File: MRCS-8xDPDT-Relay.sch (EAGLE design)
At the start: 19 parts, among them CON1 CONNECTOR-M10LOCK, K1 RELAY-G2R2, K2 RELAY-G2R2, K3 RELAY-G2R2, K4 RELAY-G2R2, K5 RELAY-G2R2, K6 RELAY-G2R2, K7 RELAY-G2R2, K8 RELAY-G2R2

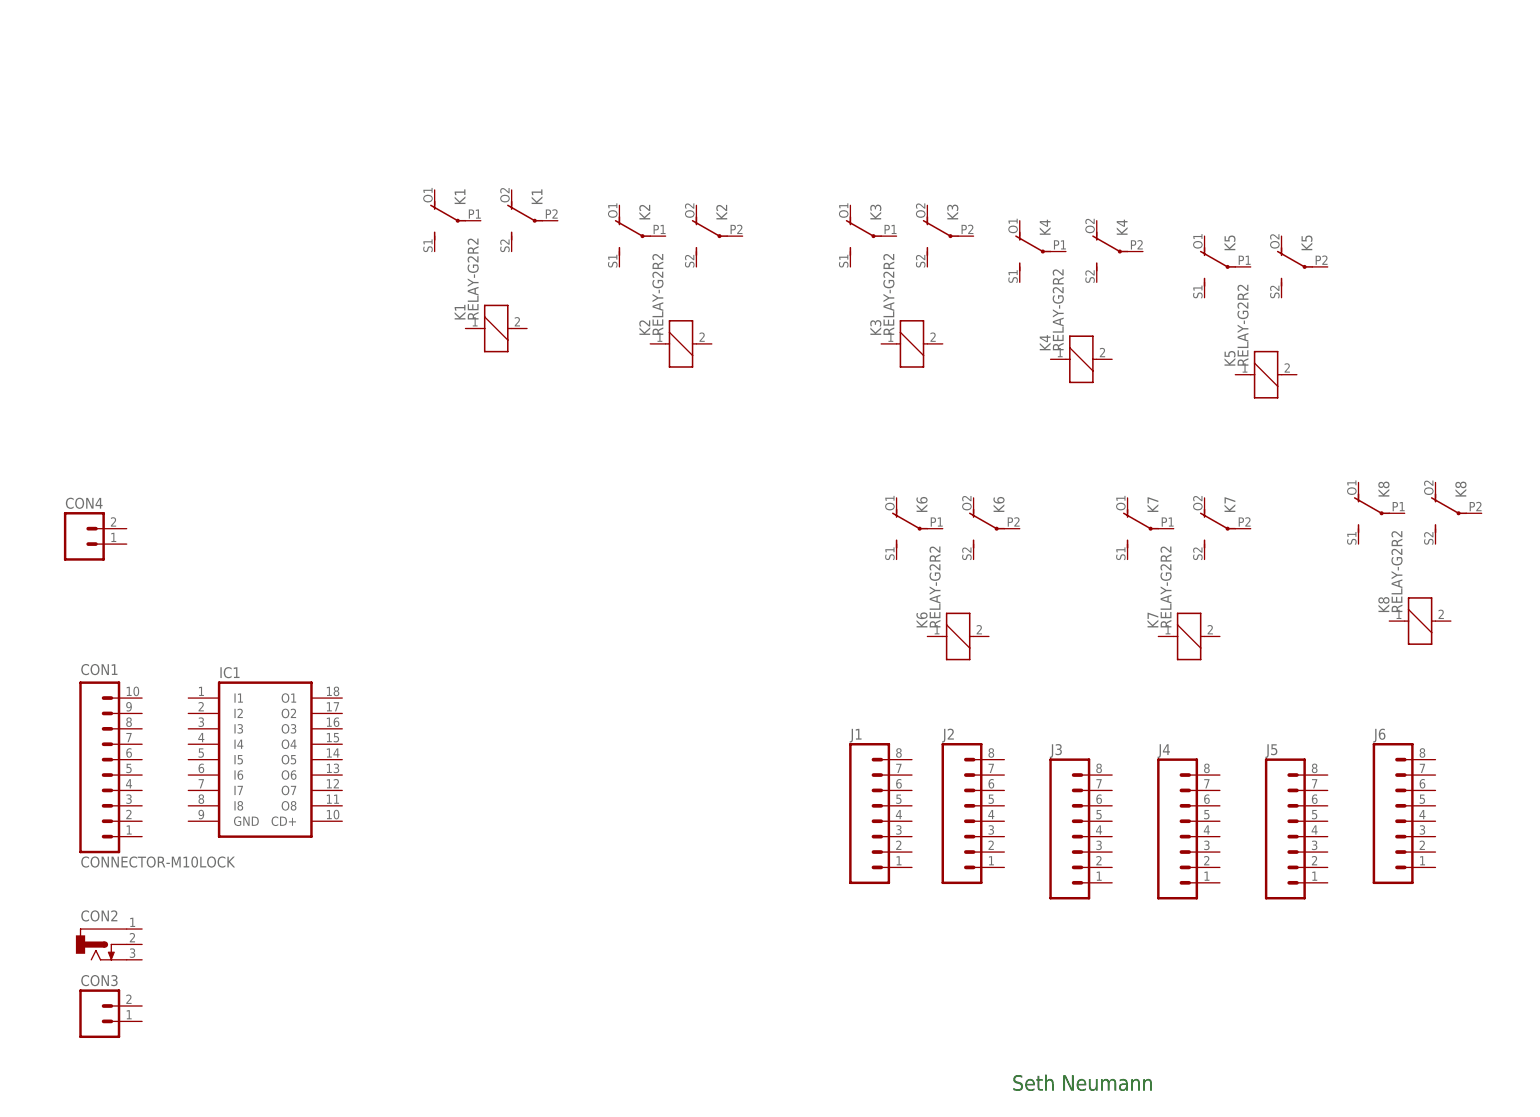
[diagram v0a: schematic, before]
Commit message: early doodling
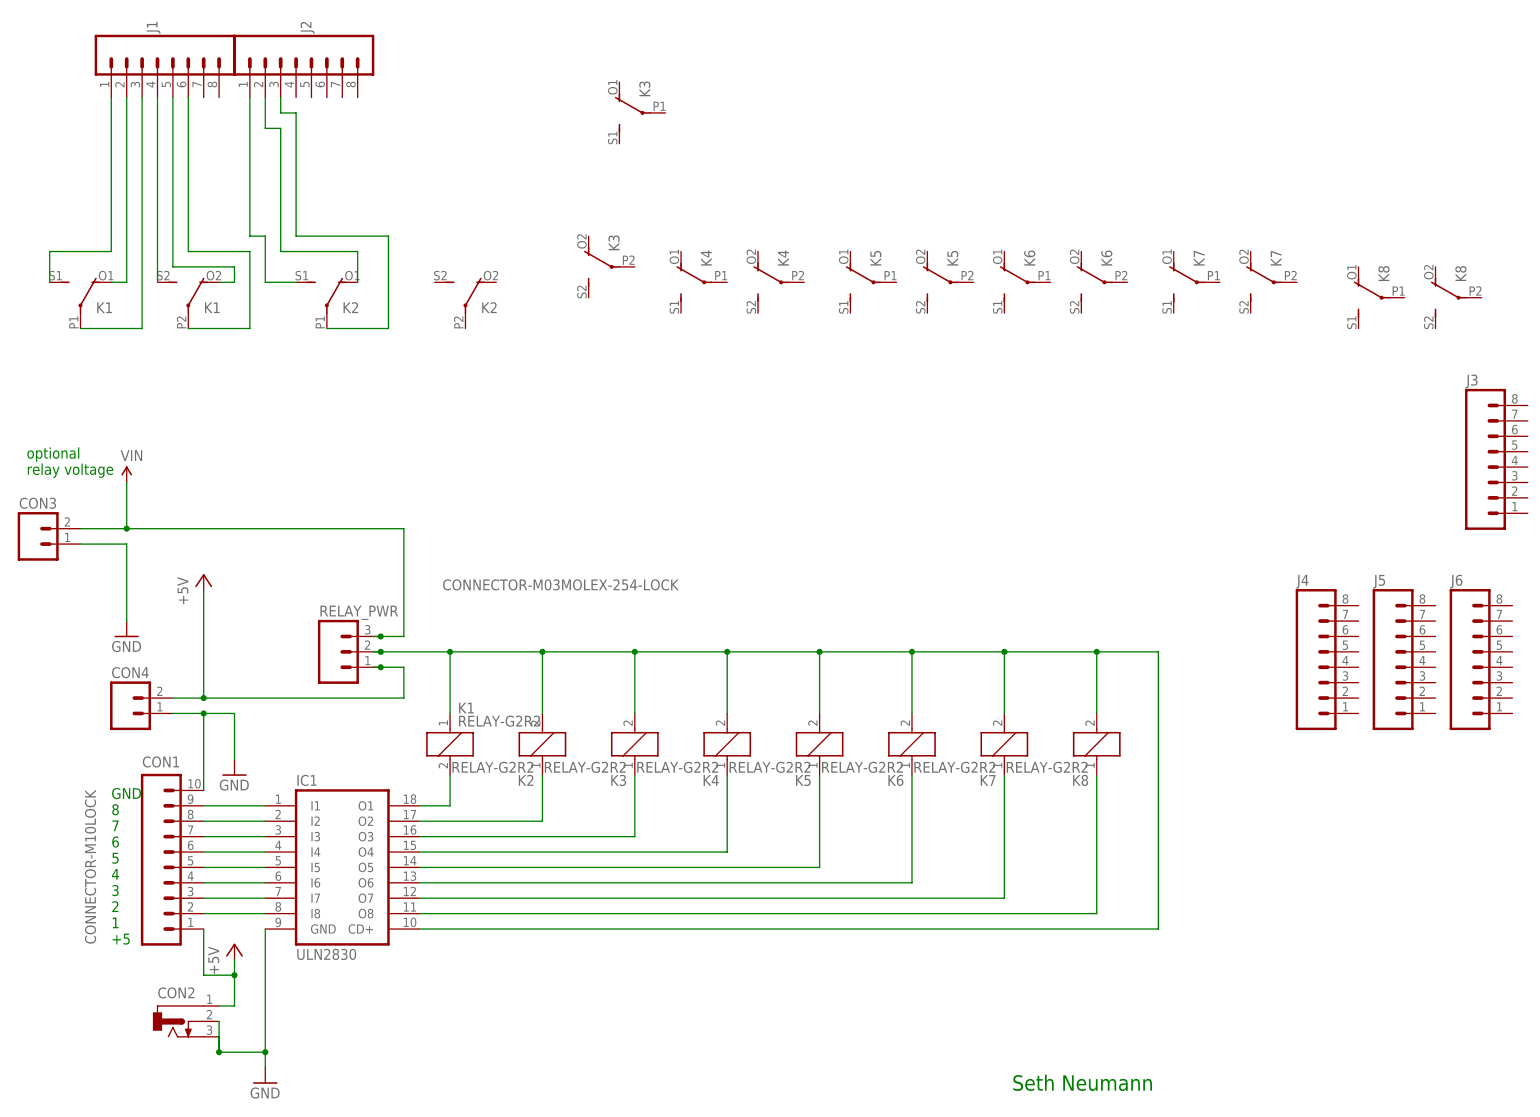
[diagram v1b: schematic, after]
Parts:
- added RELAY_PWR: CONNECTOR-M03MOLEX-254-LOCK, SPCoast:CONNECTOR-M03MOLEX-254-LOCK
- IC1: value (none) -> ULN2830
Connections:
- new net +5V: CON1.1, CON2.1, CON4.B, RELAY_PWR.1
- new net GND: CON1.10, CON2.2, CON2.3, CON3.A, CON4.A, IC1.GND
- new net N$1: CON1.9, IC1.I1
- new net N$10: IC1.O3, K31.1
- new net N$11: IC1.O4, K41.1
- new net N$12: IC1.O5, K51.1
- new net N$13: IC1.O1, K11.2
- new net N$14: IC1.O6, K61.1
- new net N$15: IC1.O7, K71.1
- new net N$16: IC1.O8, K81.1
- new net N$17: IC1.CD+, K11.1, K21.2, K31.2, K41.2, K51.2, K61.2, K71.2, K81.2, RELAY_PWR.2
- new net N$18: J1.1, K12.S
- new net N$19: J1.2, K12.O
- new net N$2: CON1.8, IC1.I2
- new net N$20: J1.3, K12.P
- new net N$21: J1.4, K13.S
- new net N$22: J1.5, K13.O
- new net N$23: J1.6, K13.P
- new net N$24: J2.1, K22.S
- new net N$25: J2.2, K22.O
- new net N$27: J2.3, K22.P
- new net N$3: CON1.7, IC1.I3
- new net N$4: CON1.6, IC1.I4
- new net N$5: CON1.5, IC1.I5
- new net N$6: CON1.4, IC1.I6
- new net N$7: CON1.3, IC1.I7
- new net N$8: CON1.2, IC1.I8
- new net N$9: IC1.O2, K21.1
- new net VIN: CON3.B, RELAY_PWR.3
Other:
- note added: "GND 8 7 6 5 4 3 2 1 +5"
- note added: "optional relay voltage"
- moved on the sheet: CON1, CON2, CON3, CON4, IC1, J1, J2, J3, J4, J5, J6, K1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

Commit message: keeping Jon up to date
adding contacts
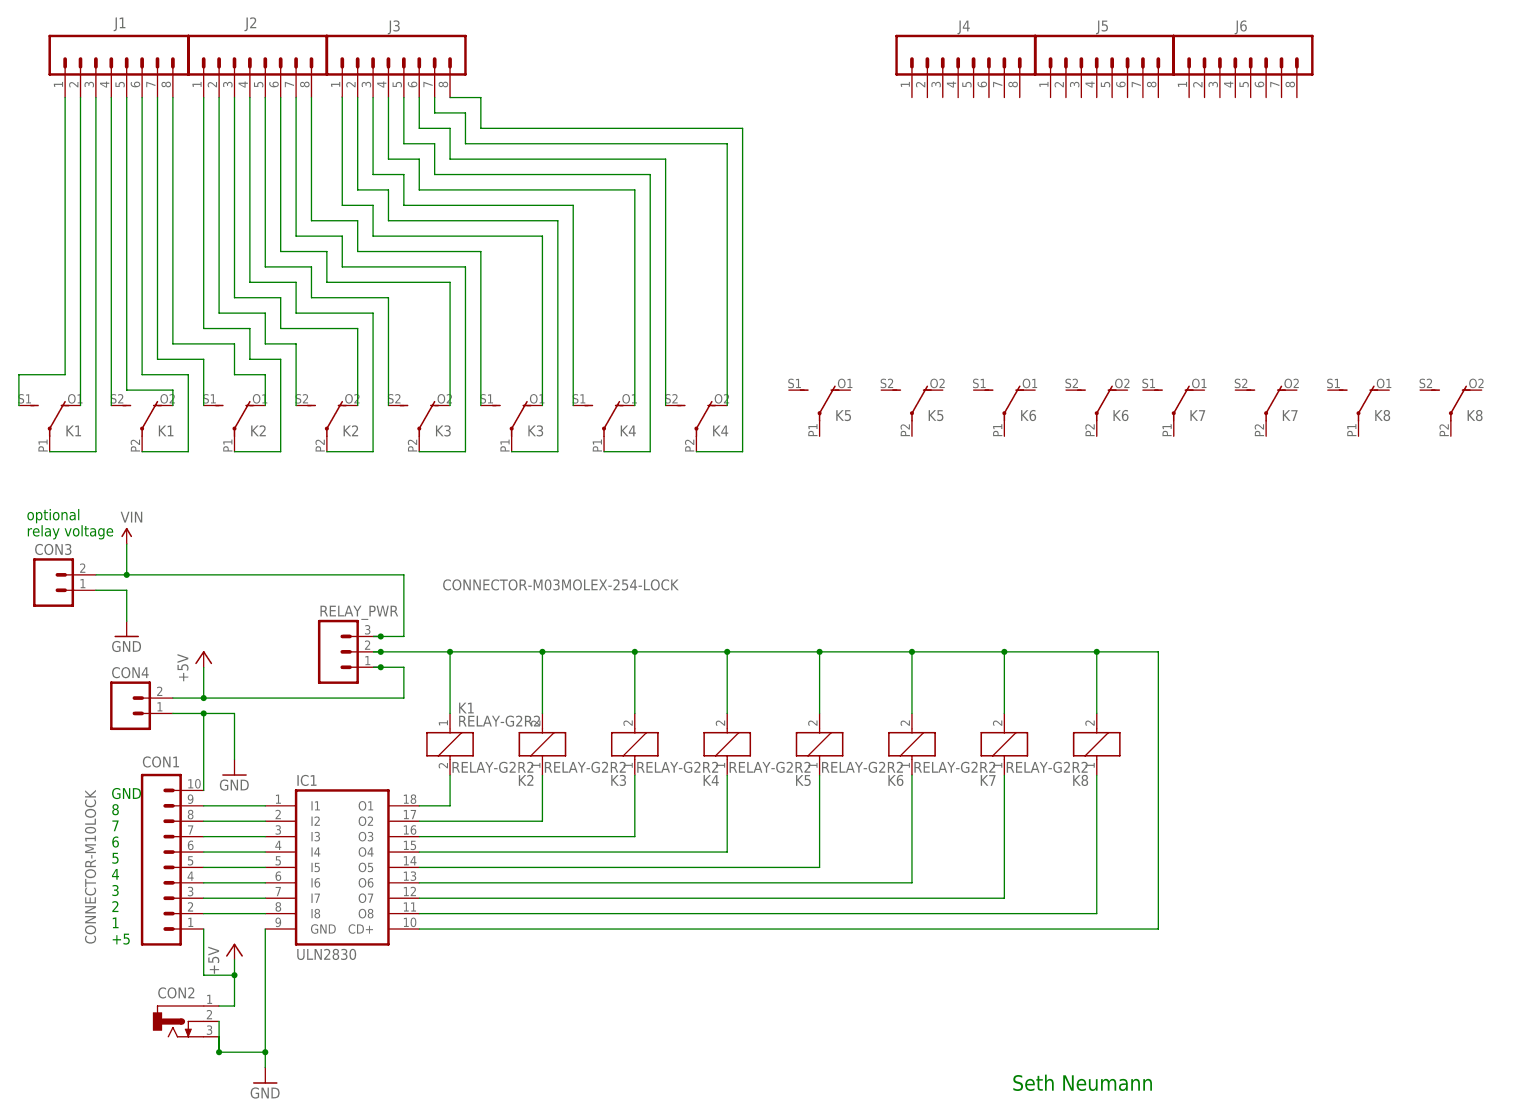
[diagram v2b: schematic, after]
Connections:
- new net N$26: J2.1, K22.P
- new net N$28: J2.3, K23.O
- new net N$29: J2.4, K23.P
- new net N$30: J2.7, K33.P
- new net N$31: J2.6, K33.O
- new net N$32: J2.8, K32.S
- new net N$33: J2.5, K33.S
- new net N$34: J3.1, K32.O
- new net N$35: J3.2, K32.P
- new net N$36: J3.3, K42.S
- new net N$37: J3.4, K42.O
- new net N$38: J3.5, K42.P
- new net N$39: J3.6, K43.S
- new net N$40: J3.7, K43.O
- new net N$41: J3.8, K43.P
- net N$24: now also J1.7; no longer J2.1
- net N$25: now also J1.8; no longer J2.2
- net N$27: now also J2.2, K23.S; no longer J2.3, K22.P
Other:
- moved on the sheet: CON3, J1, J2, J3, J4, J5, J6, K1, K2, K3, K4, K5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
